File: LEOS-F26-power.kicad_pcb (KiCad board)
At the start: 4 copper layers, 100 x 100 mm, 63 parts, among them J1 MicroFit_1x4, J2 MicroFit_1x4, J3 XT60IPW-M, J4 5V, J5 5V, J6 5V, J7 1-18V, J8 1-18V, J9 1-18V, U1 MCP2518FD, U2 MCP2562FD, U3 TPS54540BDDA, U4 TPS16630PWPR, U5 TPS54540BDDA, U6 MCP41100T-I/SN, Y1 40 MHz

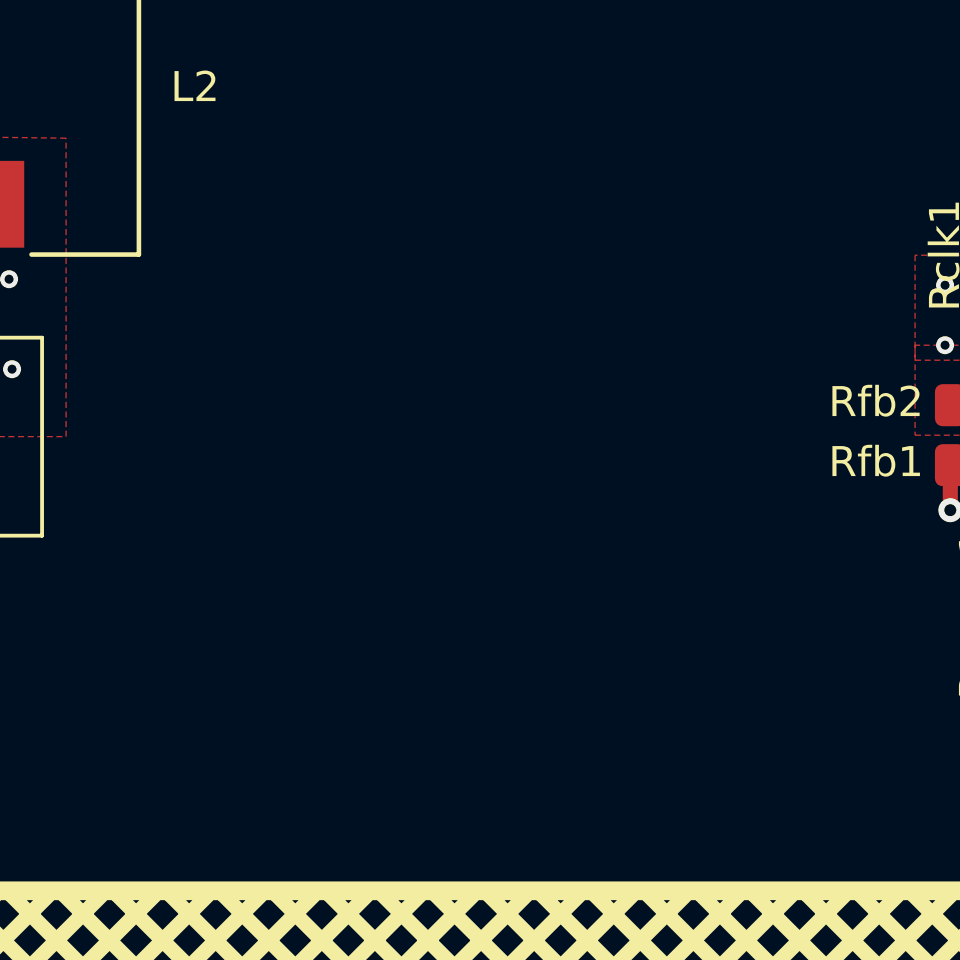
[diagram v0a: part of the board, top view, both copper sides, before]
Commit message: ewqrngfhmhgWDFEGRHTY
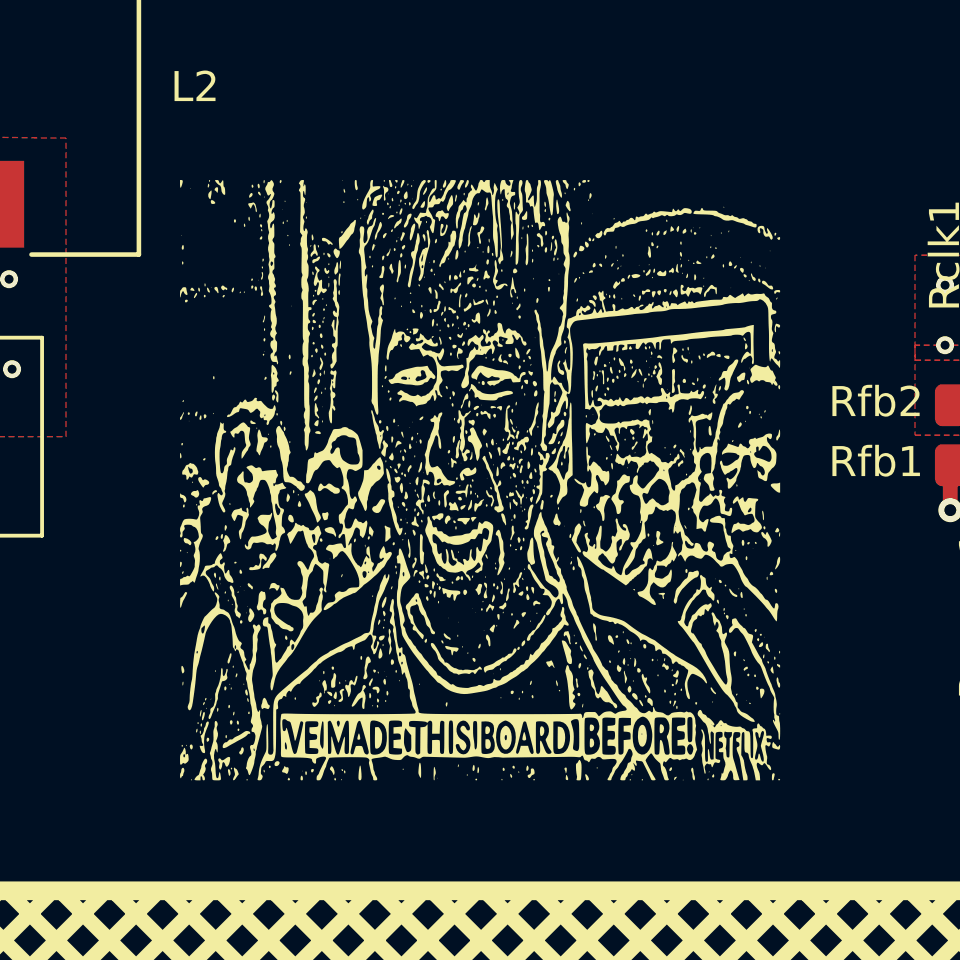
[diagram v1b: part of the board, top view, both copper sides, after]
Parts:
- added G***: LOGO, LOGO, F.Cu at (141.5, 131.5)

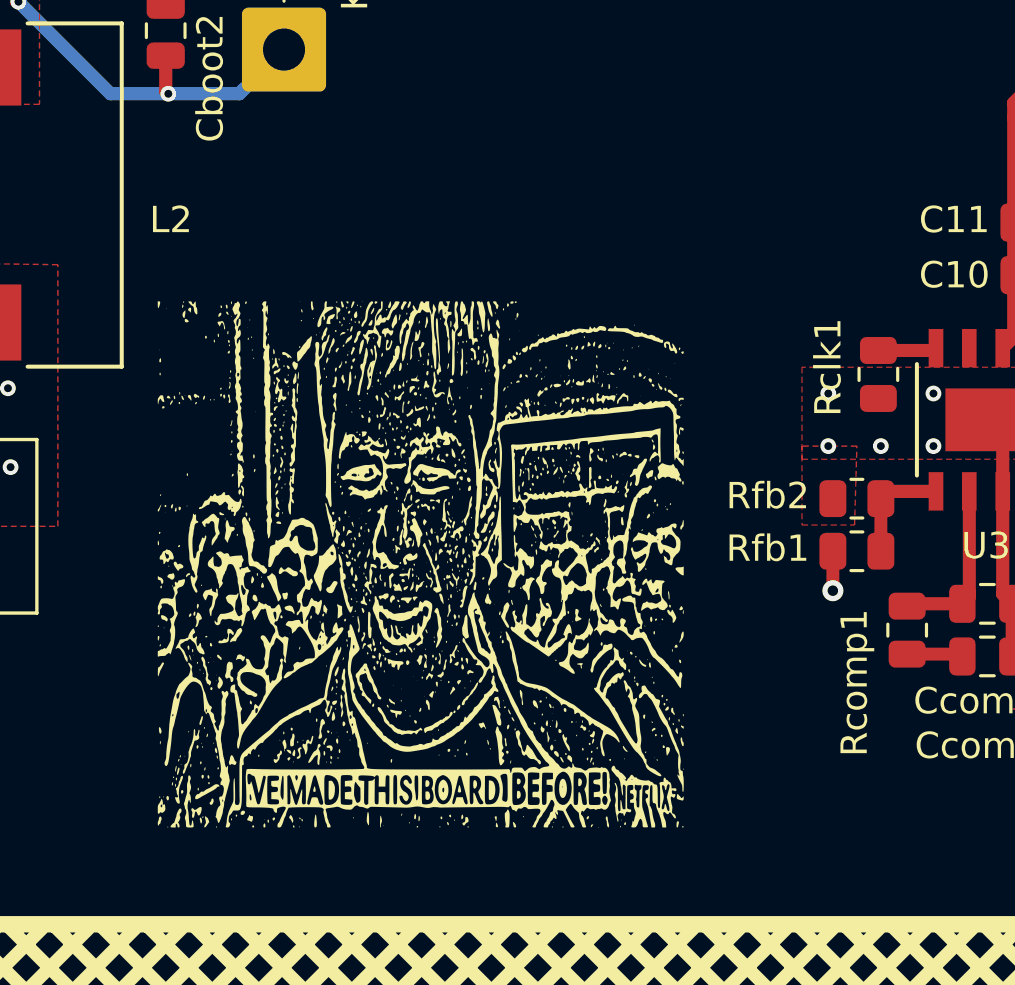
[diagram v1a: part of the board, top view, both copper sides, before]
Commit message: PLEASE SPEED I NEED THIS
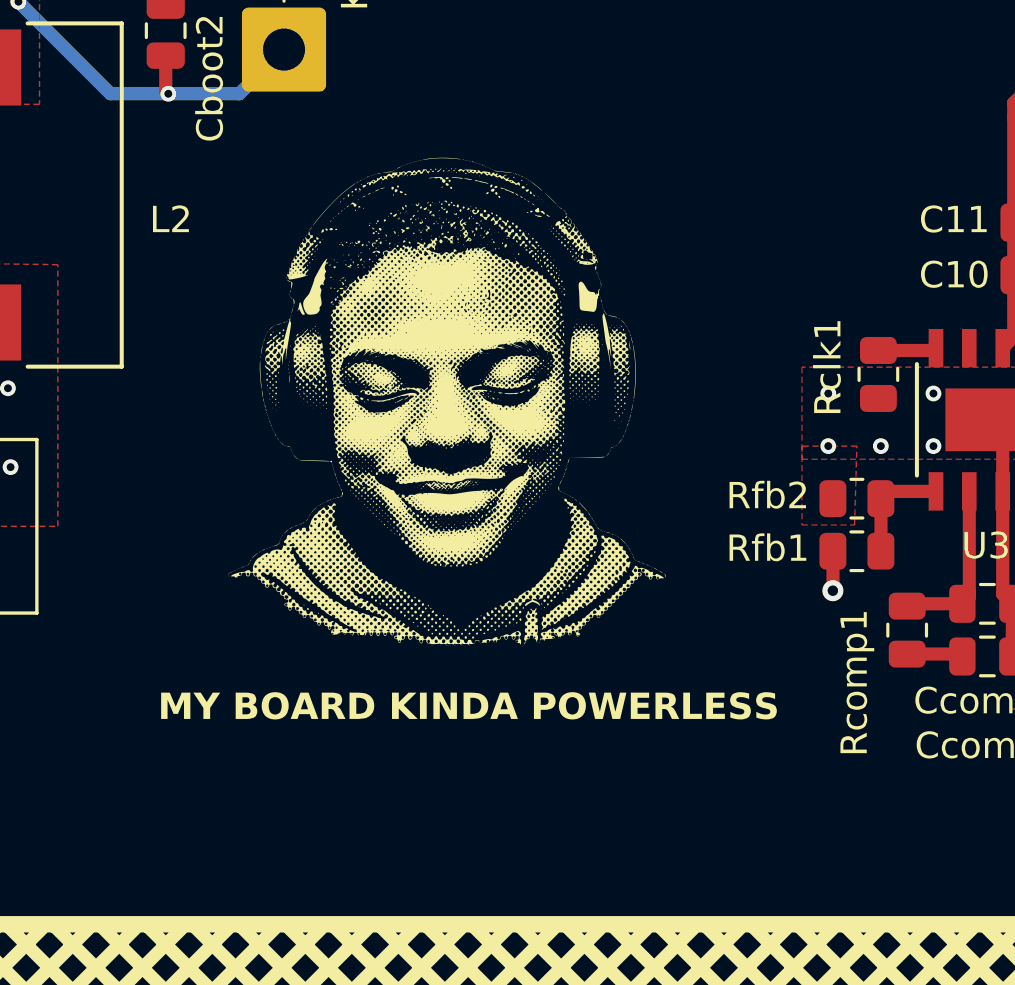
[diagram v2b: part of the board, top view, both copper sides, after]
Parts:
- moved G*** 6.08 mm to (142.5, 125.5)
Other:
- board text added: "MY BOARD KINDA POWERLESS"
